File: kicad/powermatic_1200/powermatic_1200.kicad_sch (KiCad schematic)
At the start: 62 parts, among them J1 T4171310004-001, J2 3PH-4W-PLUG, J3 BNSPDX-23-W, J4 BSPDX-23-W, J5 BSPBX-22-W, K1 HMC-9B30-11-DS, K2 HMC-9B30-11-DS, K3 HC3096N-52-900-24, K4 HMC-9B30-11-DS, K5 HMC-9B30-11-DS, K6 HMC-9B30-11-DS, M1 PWRM1200-MOTOR, Q1 FAZ-D4/2-NA-L, SW1 222102

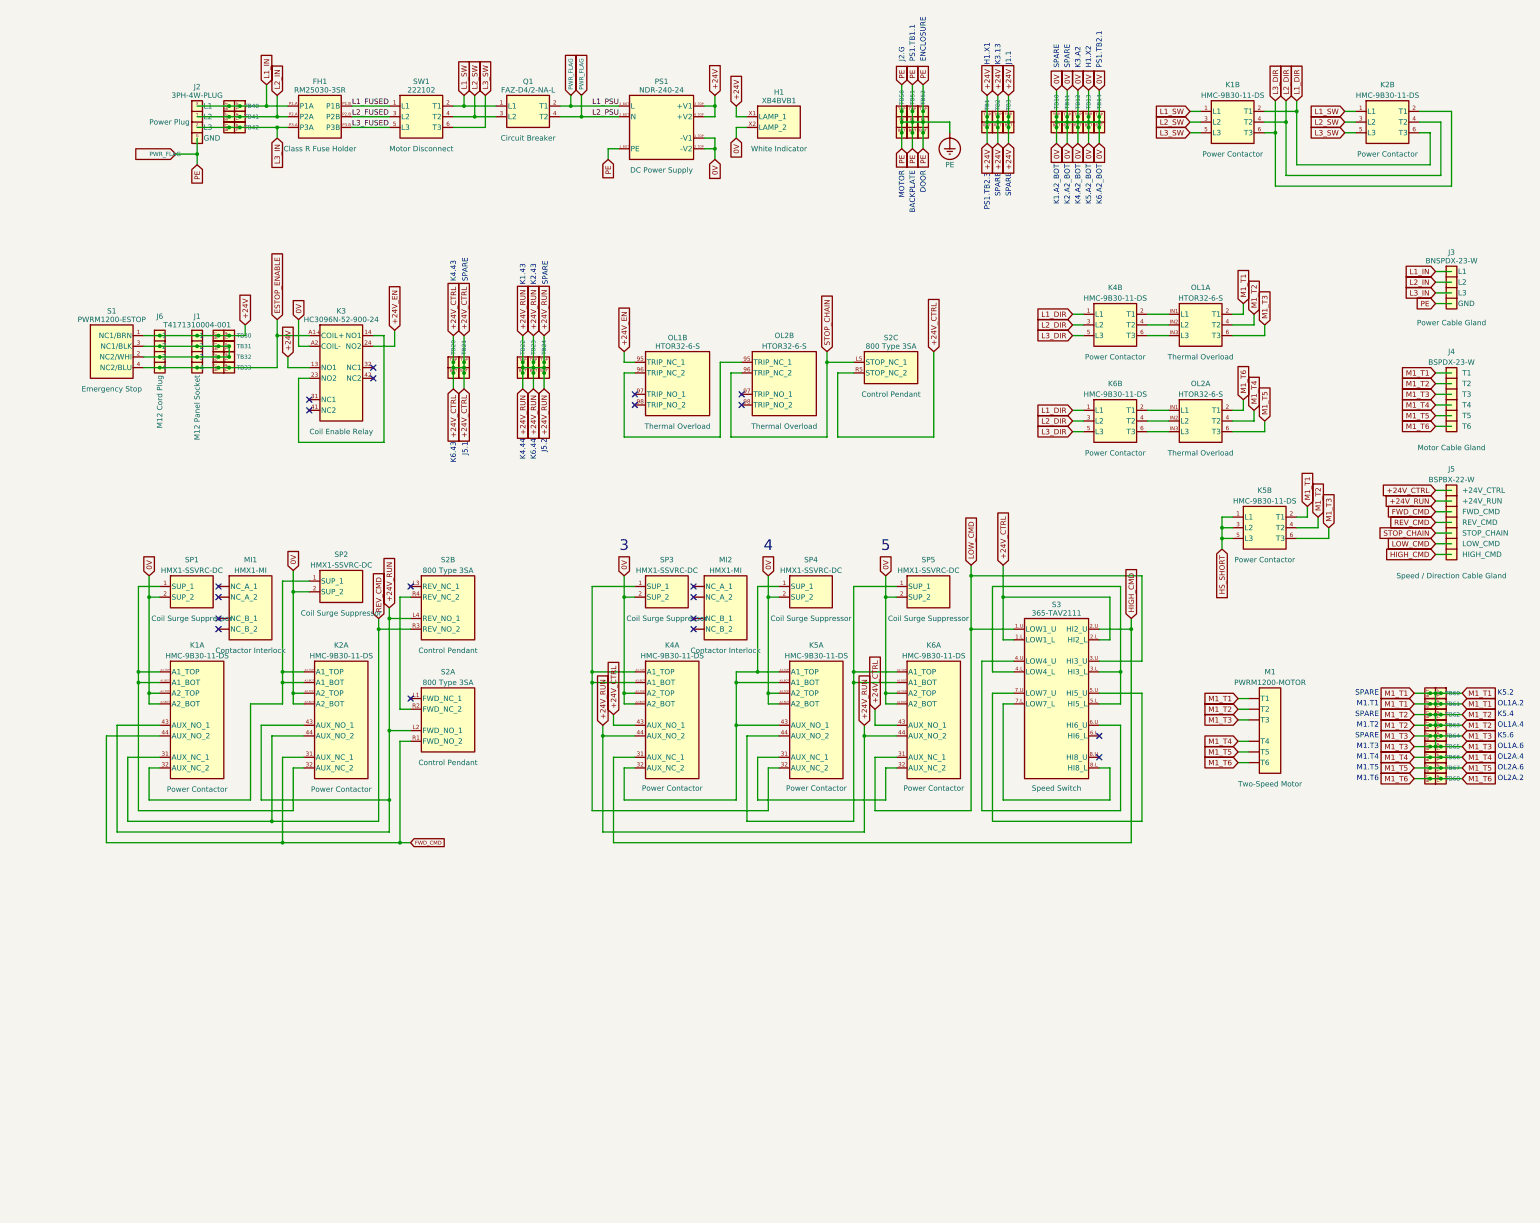
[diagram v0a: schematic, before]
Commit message: massage schematic for understanding
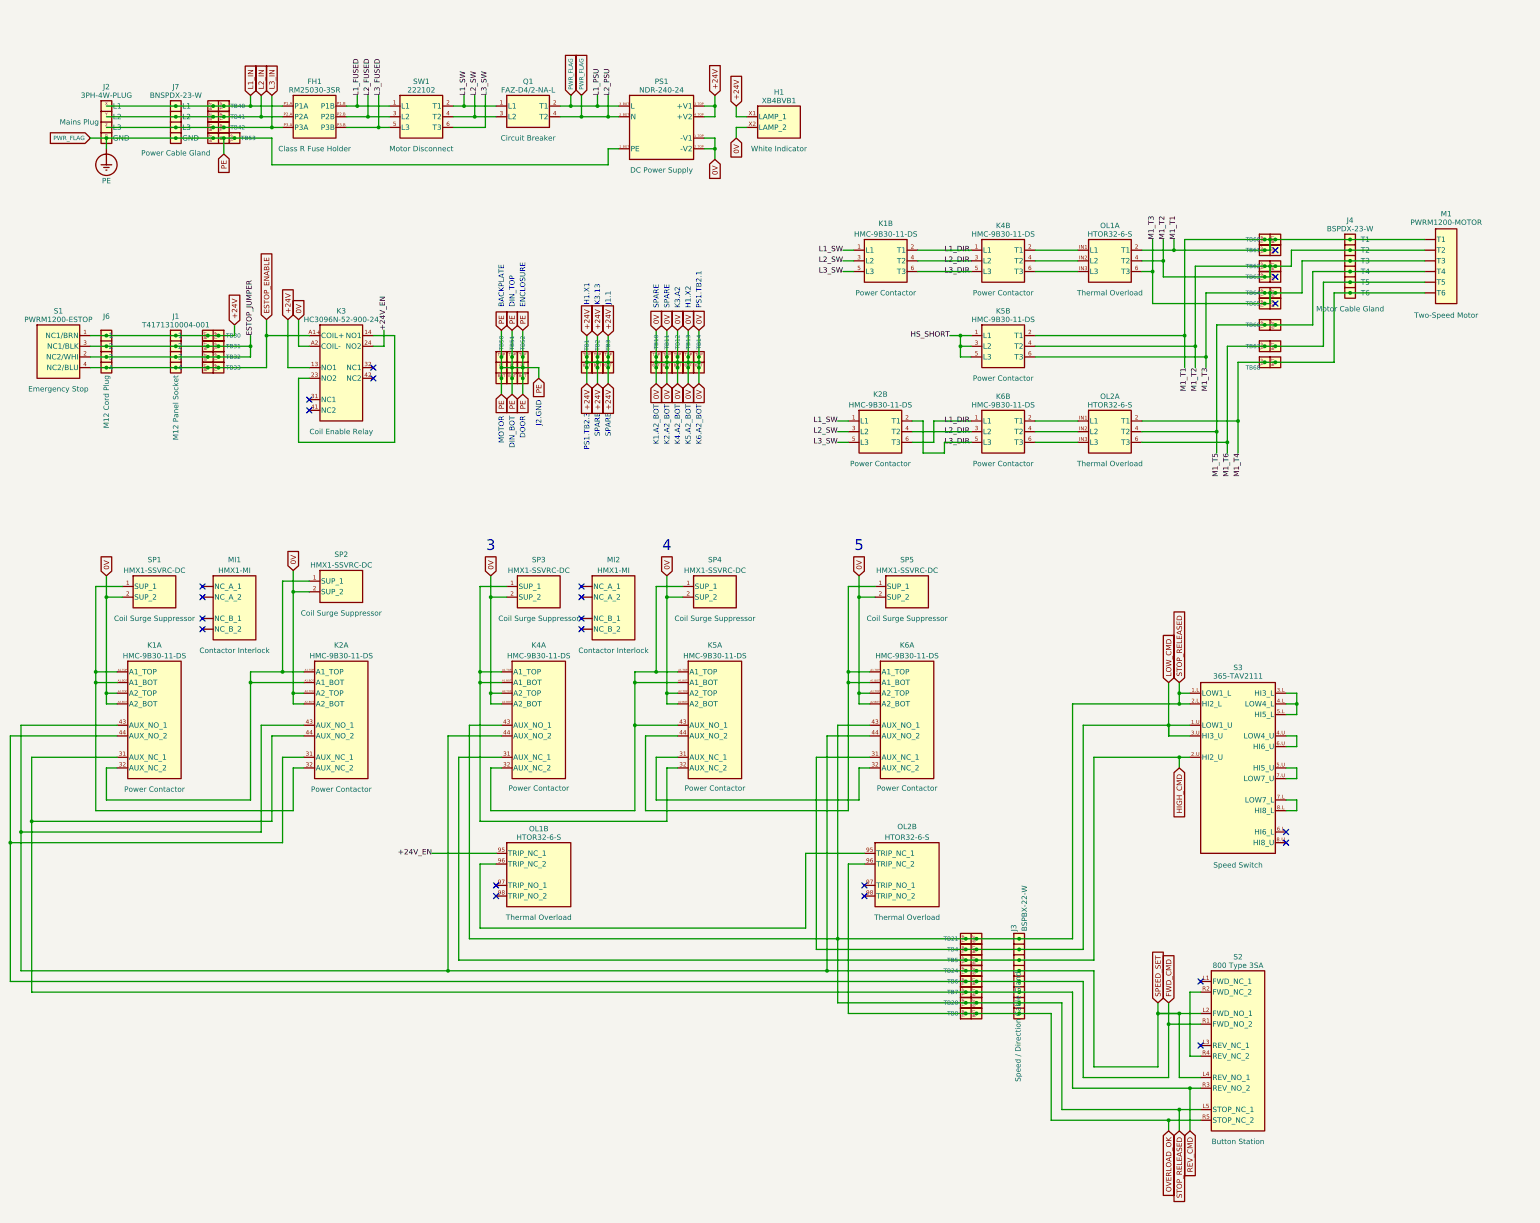
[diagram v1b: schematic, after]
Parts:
- removed J3: BNSPDX-23-W, Controls:BNSPDX-23-W_BottomWall, symbol Controls:BNSPDX-23-W
- removed J5: BSPBX-22-W, Controls:BSPBX-22-W_BottomWall, symbol Controls:BSPBX-22-W
- removed S2: 800 Type 3SA, symbol non_lcsc_parts:Non-LCSC/800S-3SA
- removed S3: 365-TAV2111, symbol non_lcsc_parts:Non-LCSC/365-TAV2111
- removed TB22, TB23: KN-T12GRY-25, Controls:KN-T12GRY-25_Front, symbol Controls:KN-T12GRY-25
- added J3: BSPBX-22-W, Controls:BSPBX-22-W_BottomWall, symbol non_lcsc_parts:Non-LCSC/BSPBX-22-W
- added J7: BNSPDX-23-W, Controls:BNSPDX-23-W_BottomWall, symbol Controls:BNSPDX-23-W
- added S2: 800 Type 3SA, symbol Controls:800S-3SA
- added S3: 365-TAV2111, symbol Controls:365-TAV2111
- added TB4, TB5, TB6, TB7, TB8: KN-T12GRY-25, Controls:KN-T12GRY-25_Front, symbol Controls:KN-T12GRY-25
- added TB53: KN-G12SP-10, Controls:KN-G12SP-10_Front, symbol Controls:KN-G12SP-10
- J2: Part Name Power Plug -> Mains Plug
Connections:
- net FWD_CMD: now also J3.5, S2.R1 (FWD_NO_2), TB6.BOT (TERM), TB6.TOP (TERM)
- net HIGH_CMD: now also J3.3, S3.2.U (HI2_U), TB5.BOT (TERM), TB5.TOP (TERM)
- net L1_IN: now also J7.X (L1)
- net L2_IN: now also J7.Y (L2)
- net L3_IN: now also J7.Z (L3)
- net LOW_CMD: now also J3.2, S3.1.U (LOW1_U), S3.3.U (HI3_U), TB4.BOT (TERM), TB4.TOP (TERM)
- net M1_T1: no longer TB61.BOT (TERM)
- net M1_T2: no longer TB63.BOT (TERM)
- net M1_T3: no longer TB65.BOT (TERM)
- net M1_T4: now also J4.T6, M1.T6, OL2.2 (T1), TB68.BOT (TERM), TB68.TOP (TERM); no longer J4.T4, M1.T4, OL2.4 (T2), TB66.BOT (TERM), TB66.TOP (TERM)
- net M1_T5: now also J4.T4, M1.T4, OL2.4 (T2), TB66.BOT (TERM), TB66.TOP (TERM); no longer J4.T5, M1.T5, OL2.6 (T3), TB67.BOT (TERM), TB67.TOP (TERM)
- net M1_T6: now also J4.T5, M1.T5, OL2.6 (T3), TB67.BOT (TERM), TB67.TOP (TERM); no longer J4.T6, M1.T6, OL2.2 (T1), TB68.BOT (TERM), TB68.TOP (TERM)
- net PE: now also J7.G (GND), TB53.BOT (TERM), TB53.PE, TB53.TOP (TERM)
- net REV_CMD: now also J3.6, S2.R3 (REV_NO_2), TB7.BOT (TERM), TB7.TOP (TERM)
- net ESTOP_JUMPER: now reaches J1.2, J1.3, J6.2, J6.3, S1.2 (NC2/WHI), S1.3 (NC1/BLK), TB31.BOT (TERM), TB31.TOP (TERM), TB32.BOT (TERM), TB32.TOP (TERM)
- net +24V_CTRL renamed STOP_RELEASED
- net STOP_RELEASED: now also J3.1, J3.7 (8), S2.L5 (STOP_NC_1), S3.1.L (LOW1_L), S3.2.L (HI2_L)
- net +24V_RUN renamed SPEED_SET
- net SPEED_SET: now also J3.4, S2.L2 (FWD_NO_1), S2.L4 (REV_NO_1)
- net STOP_CHAIN renamed OVERLOAD_OK
- net OVERLOAD_OK: now also J3.7 (8), S2.R5 (STOP_NC_2), TB8.BOT (TERM), TB8.TOP (TERM)
- new net: S3.3.L (HI3_L), S3.4.L (LOW4_L), S3.5.L (HI5_L)
- new net: S3.4.U (LOW4_U), S3.6.U (HI6_U)
- new net: S3.5.U (HI5_U), S3.7.U (LOW7_U)
- new net: S3.7.L (LOW7_L), S3.8.L (HI8_L)
- new net: S2.R2 (FWD_NC_2), S2.R4 (REV_NC_2)
- no-connect marks 20 -> 23
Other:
- note added: "DIN_BOT"
- note added: "DIN_TOP"
- note added: "J2.GND"
- note removed: "J2.G"
- note removed: "J5.1"
- note removed: "J5.2"
- note removed: "K1.43"
- note removed: "K2.43"
- note removed: "K4.43"
- note removed: "K4.44"
- note removed: "K5.2"
- note removed: "K5.4"
- note removed: "K5.6"
- note removed: "K6.43"
- note removed: "K6.44"
- note removed: "M1.T1"
- note removed: "M1.T2"
- note removed: "M1.T3"
- note removed: "M1.T4"
- note removed: "M1.T5"
- note removed: "M1.T6"
- note removed: "OL1A.2"
- note removed: "OL1A.4"
- note removed: "OL1A.6"
- note removed: "OL2A.2"
- note removed: "OL2A.4"
- note removed: "OL2A.6"
- note removed: "PS1.TB1.1"
- moved on the sheet: FH1, J1, J2, J4, J6, K1A, K2B, K4A, K4B, K5A, K5B, K6A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
